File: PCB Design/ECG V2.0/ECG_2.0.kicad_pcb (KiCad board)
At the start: 4 copper layers, 42.3 x 69.7 mm, 50 parts, among them J1 01x05_Female, J2 JST_01x04_Male, U1 Li-Po, U10 ESP32-C3-MINI-1-N4, U11 FS8205A, U12 DW01, U2 TP4056-C21417, U3 USBLC6-2SC6, U4 Battery_Switch, U5 5V_switch, U6 TLV62568DBV, U7 MCU_switch, U8 Tactile_push_button_6x6mm, U9 USB-TYPE0-C-16P

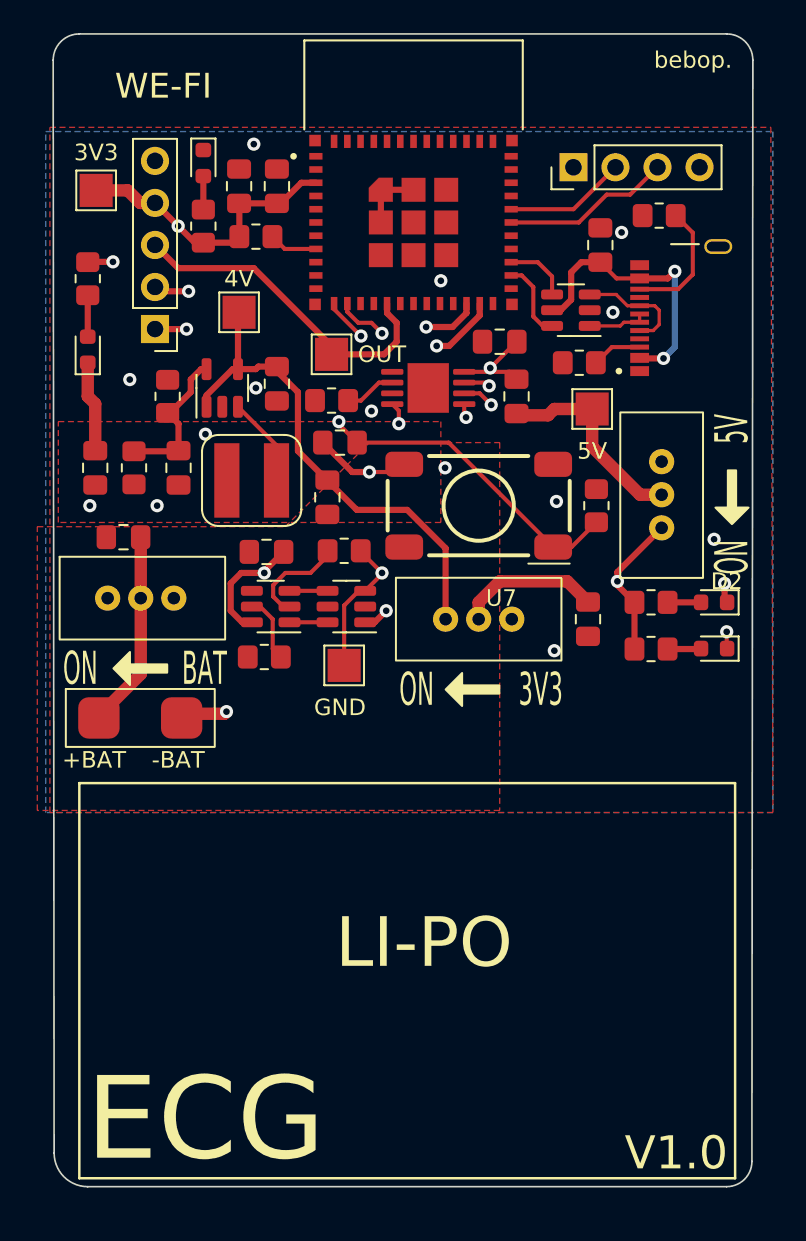
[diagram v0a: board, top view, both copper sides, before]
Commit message: Improved PCB design and Improved renderings
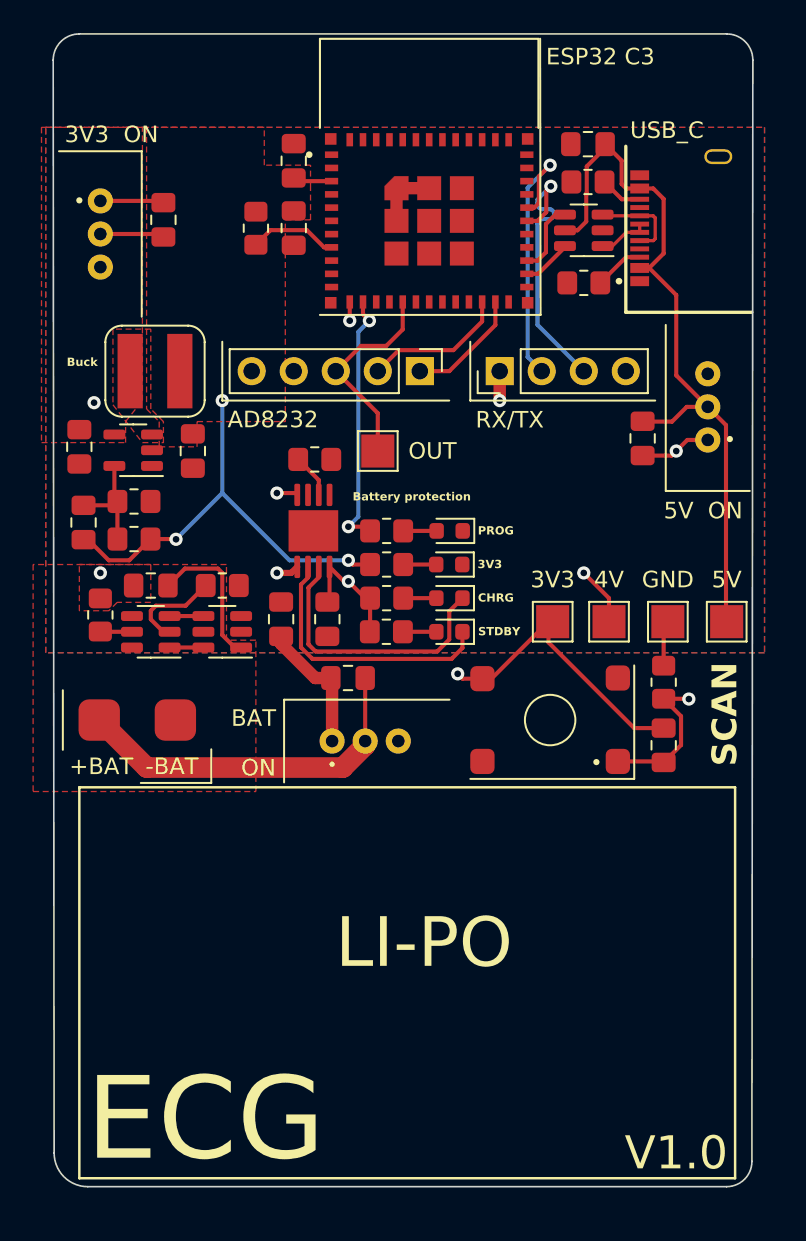
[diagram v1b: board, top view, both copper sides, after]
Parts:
- moved 3V3 37.9 mm to (160.2, 102.5)
- moved U7 32.6 mm to (132.8, 79.1), turned to -90 degrees
- moved 4V 29.1 mm to (163.6, 102.5)
- moved D4 28.4 mm to (153.9, 99.1), turned to 180 degrees
- moved C1 26.8 mm to (166.9, 110.0), turned to -90 degrees
- moved D3 24.5 mm to (153.9, 97.0), turned to 180 degrees
- moved R4 23.6 mm to (150.1, 97.0), turned to 0 degrees
- moved R7 23.3 mm to (150.1, 99.1), turned to 0 degrees
- moved GND 19.7 mm to (167.1, 102.5)
- moved C3 19.7 mm to (146.6, 102.4), turned to -90 degrees
- moved C13 19.5 mm to (136.7, 78.2)
- moved C2 18.5 mm to (143.8, 102.4), turned to 90 degrees
- moved J1 16.2 mm to (152.1, 87.4), turned to -90 degrees
- moved U4 16.1 mm to (148.8, 109.7)
- moved R3 16.0 mm to (150.1, 103.1)
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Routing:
- net +3V3: track 23.1 -> 71.7 mm
- net BTN: track 27.8 -> 44.0 mm
- net +LO: track 22.4 -> 7.11 mm, vias 2 -> 0
- net -LO: track 21.9 -> 8.73 mm, vias 2 -> 0
- net GND: track 18.1 -> 6.61 mm, vias 11 -> 0
- net +4V: track 30.4 -> 41.3 mm, vias 0 -> 2
- net BatO: track 11.7 -> 21.9 mm
- net /TX: track 7.35 -> 16.8 mm, vias 0 -> 1
- net Output: track 20.5 -> 12.6 mm
- net Net-(D2-Pad1): track 23.9 -> 16.3 mm, vias 2 -> 0
- net LED: track 22.8 -> 15.7 mm
- net /RX: track 10.2 -> 17.2 mm, vias 0 -> 1
- net Net-(D1-Pad1): track 23.2 -> 16.8 mm, vias 2 -> 0
- net In_5V: track 39.2 -> 44.9 mm, vias 2 -> 0
- net Net-(L1-Pad1): track 5.41 -> 0.00 mm
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- added copper zone on F.Cu, net +4V
- added copper zone on In1.Cu, net +BATT
- added copper zone on F.Cu, net Net-(L1-Pad1)
- added copper zone on F.Cu, net VSS
- removed copper zone on In1.Cu, net +3V3
- removed copper zone on In1.Cu, net VSS
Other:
- board text added: "3V3"
- board text added: "Battery protection"
- board text added: "Buck"
- board text added: "PROG"
- board text added: "SCAN"
- board text added: "STDBY"
- board text removed: "WE-FI"
- board text removed: "bebop."
